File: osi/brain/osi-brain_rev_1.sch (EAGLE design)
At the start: 8 parts, among them IC1 TINY24/44/84-PU

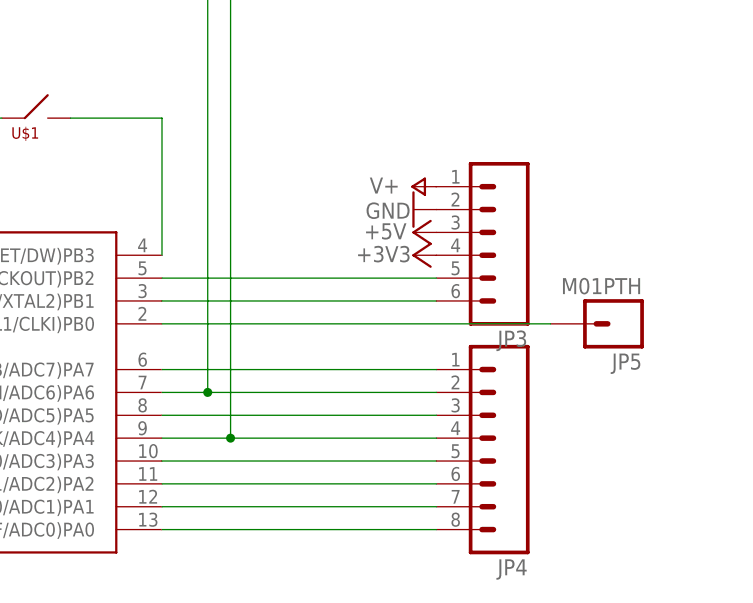
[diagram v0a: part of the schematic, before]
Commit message: power-ac
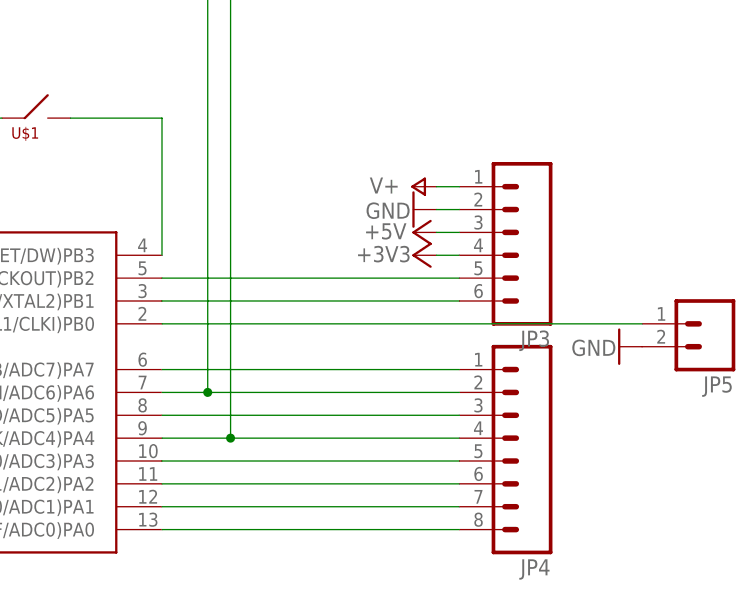
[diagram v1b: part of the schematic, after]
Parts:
- JP3: device SparkFun_mod:M06SIP -> SparkFun:M06SIP
- JP4: device SparkFun_mod:M081X08 -> SparkFun:M081X08
- JP5: value M01PTH -> (none); device SparkFun_mod:M01PTH -> SparkFun_mod:M021X02_NO_SILK
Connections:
- net GND: now also JP5.2
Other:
- moved on the sheet: JP3, JP4
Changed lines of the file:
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@@
 <part name="GND2" library="SparkFun" deviceset="GND" device=""/>
 <part name="GND5" library="SparkFun" deviceset="GND" device=""/>
-<part name="JP3" library="SparkFun_mod" deviceset="M06" device="SIP"/>
-<part name="JP4" library="SparkFun_mod" deviceset="M08" device="1X08"/>
 <part name="GND4" library="SparkFun" deviceset="GND" device=""/>
 <part name="P+2" library="supply1" deviceset="V+" device=""/>
@@
 <part name="JP2" library="SparkFun_mod" deviceset="M05" device="PTH"/>
 <part name="P+4" library="supply1" deviceset="+5V" device=""/>
-<part name="JP5" library="SparkFun_mod" deviceset="M01" device="PTH"/>
 <part name="+3V2" library="supply1" deviceset="+3V3" device=""/>
+<part name="JP3" library="SparkFun" deviceset="M06" device="SIP"/>
+<part name="JP4" library="SparkFun" deviceset="M08" device="1X08"/>
+<part name="GND3" library="SparkFun" deviceset="GND" device=""/>
+<part name="JP5" library="SparkFun_mod" deviceset="M02" device="1X02_NO_SILK"/>
 </parts>
 <sheets>
@@
 <attribute name="VALUE" x="111.506" y="67.564" size="1.778" layer="96"/>
 </instance>
-<instance part="JP3" gate="G$1" x="124.46" y="66.04" rot="R180"/>
-<instance part="JP4" gate="G$1" x="124.46" y="43.18" rot="R180"/>
 <instance part="GND4" gate="1" x="93.98" y="121.92" rot="R180"/>
 <instance part="P+2" gate="1" x="116.84" y="71.12" smashed="yes" rot="R90">
@@
 <attribute name="VALUE" x="105.156" y="122.682" size="1.778" layer="96" rot="R90"/>
 </instance>
-<instance part="JP5" gate="G$1" x="139.7" y="55.88" rot="R180"/>
 <instance part="+3V2" gate="G$1" x="22.86" y="45.72" smashed="yes" rot="R90">
 <attribute name="VALUE" x="22.606" y="46.736" size="1.778" layer="96" rot="R180"/>
 </instance>
+<instance part="JP3" gate="G$1" x="127" y="66.04" rot="R180"/>
+<instance part="JP4" gate="G$1" x="127" y="43.18" rot="R180"/>
+<instance part="GND3" gate="1" x="139.7" y="53.34" smashed="yes" rot="R270">
+<attribute name="VALUE" x="134.366" y="52.324" size="1.778" layer="96"/>
+</instance>
+<instance part="JP5" gate="G$1" x="149.86" y="55.88" rot="R180"/>
 </instances>
 <busses>
@@
 </segment>
 <segment>
+<pinref part="GND5" gate="1" pin="GND"/>
+<wire x1="121.92" y1="68.58" x2="119.38" y2="68.58" width="0.1524" layer="91"/>
 <pinref part="JP3" gate="G$1" pin="2"/>
-<pinref part="GND5" gate="1" pin="GND"/>
+</segment>
+<segment>
+<pinref part="GND3" gate="1" pin="GND"/>
+<pinref part="JP5" gate="G$1" pin="2"/>
 </segment>
 </net>
@@
 <segment>
 <pinref part="IC1" gate="1" pin="(PCINT3/T0/ADC3)PA3"/>
-<wire x1="119.38" y1="40.64" x2="88.9" y2="40.64" width="0.1524" layer="91"/>
+<wire x1="121.92" y1="40.64" x2="88.9" y2="40.64" width="0.1524" layer="91"/>
 <pinref part="JP4" gate="G$1" pin="5"/>
 </segment>
@@
 <segment>
 <pinref part="IC1" gate="1" pin="(PCINT2/AIN1/ADC2)PA2"/>
-<wire x1="119.38" y1="38.1" x2="88.9" y2="38.1" width="0.1524" layer="91"/>
+<wire x1="121.92" y1="38.1" x2="88.9" y2="38.1" width="0.1524" layer="91"/>
 <pinref part="JP4" gate="G$1" pin="6"/>
 </segment>
@@
 <segment>
 <pinref part="IC1" gate="1" pin="(PCINT1/AIN0/ADC1)PA1"/>
-<wire x1="119.38" y1="35.56" x2="88.9" y2="35.56" width="0.1524" layer="91"/>
+<wire x1="121.92" y1="35.56" x2="88.9" y2="35.56" width="0.1524" layer="91"/>
 <pinref part="JP4" gate="G$1" pin="7"/>
 </segment>
@@
 <segment>
 <pinref part="IC1" gate="1" pin="(PCINT0/AREF/ADC0)PA0"/>
-<wire x1="119.38" y1="33.02" x2="88.9" y2="33.02" width="0.1524" layer="91"/>
+<wire x1="121.92" y1="33.02" x2="88.9" y2="33.02" width="0.1524" layer="91"/>
 <pinref part="JP4" gate="G$1" pin="8"/>
 </segment>
@@
 <segment>
 <wire x1="114.3" y1="109.22" x2="93.98" y2="109.22" width="0.1524" layer="91"/>
-<pinref part="JP4" gate="G$1" pin="2"/>
-<wire x1="93.98" y1="48.26" x2="119.38" y2="48.26" width="0.1524" layer="91"/>
+<wire x1="93.98" y1="48.26" x2="121.92" y2="48.26" width="0.1524" layer="91"/>
 <wire x1="93.98" y1="109.22" x2="93.98" y2="48.26" width="0.1524" layer="91"/>
 <junction x="93.98" y="48.26"/>
@@
 <pinref part="IC1" gate="1" pin="(PCINT6/OC1A/SDA/MOSI/ADC6)PA6"/>
 <wire x1="88.9" y1="48.26" x2="93.98" y2="48.26" width="0.1524" layer="91"/>
+<pinref part="JP4" gate="G$1" pin="2"/>
 </segment>
 </net>
 <net name="V+" class="0">
 <segment>
+<pinref part="P+2" gate="1" pin="V+"/>
+<wire x1="121.92" y1="71.12" x2="119.38" y2="71.12" width="0.1524" layer="91"/>
 <pinref part="JP3" gate="G$1" pin="1"/>
-<pinref part="P+2" gate="1" pin="V+"/>
 </segment>
 </net>
@@
 <segment>
 <pinref part="IC1" gate="1" pin="(PCINT5/OC1B/MISO/DO/ADC5)PA5"/>
+<wire x1="88.9" y1="45.72" x2="121.92" y2="45.72" width="0.1524" layer="91"/>
 <pinref part="JP4" gate="G$1" pin="3"/>
-<wire x1="88.9" y1="45.72" x2="119.38" y2="45.72" width="0.1524" layer="91"/>
 </segment>
 </net>
@@
 <segment>
 <wire x1="114.3" y1="106.68" x2="96.52" y2="106.68" width="0.1524" layer="91"/>
-<pinref part="JP4" gate="G$1" pin="4"/>
-<wire x1="96.52" y1="43.18" x2="119.38" y2="43.18" width="0.1524" layer="91"/>
+<wire x1="96.52" y1="43.18" x2="121.92" y2="43.18" width="0.1524" layer="91"/>
 <wire x1="96.52" y1="106.68" x2="96.52" y2="43.18" width="0.1524" layer="91"/>
 <wire x1="76.2" y1="106.68" x2="96.52" y2="106.68" width="0.1524" layer="91"/>
@@
 <wire x1="88.9" y1="43.18" x2="96.52" y2="43.18" width="0.1524" layer="91"/>
 <junction x="96.52" y="43.18"/>
+<pinref part="JP4" gate="G$1" pin="4"/>
 </segment>
 </net>
@@
 <segment>
 <pinref part="IC1" gate="1" pin="(PCINT10/INT0/OC0A/CKOUT)PB2"/>
-<wire x1="88.9" y1="60.96" x2="119.38" y2="60.96" width="0.1524" layer="91"/>
+<wire x1="88.9" y1="60.96" x2="121.92" y2="60.96" width="0.1524" layer="91"/>
 <pinref part="JP3" gate="G$1" pin="5"/>
 </segment>
@@
 <segment>
 <pinref part="IC1" gate="1" pin="(PCINT9/XTAL2)PB1"/>
-<wire x1="88.9" y1="58.42" x2="119.38" y2="58.42" width="0.1524" layer="91"/>
+<wire x1="88.9" y1="58.42" x2="121.92" y2="58.42" width="0.1524" layer="91"/>
 <pinref part="JP3" gate="G$1" pin="6"/>
 </segment>
@@
 <segment>
 <pinref part="IC1" gate="1" pin="(PCINT8/XTAL1/CLKI)PB0"/>
-<wire x1="88.9" y1="55.88" x2="132.08" y2="55.88" width="0.1524" layer="91"/>
+<wire x1="88.9" y1="55.88" x2="142.24" y2="55.88" width="0.1524" layer="91"/>
 <pinref part="JP5" gate="G$1" pin="1"/>
 </segment>
@@
 <segment>
 <pinref part="IC1" gate="1" pin="(PCINT7/ICP/OC0B/ADC7)PA7"/>
+<wire x1="88.9" y1="50.8" x2="121.92" y2="50.8" width="0.1524" layer="91"/>
 <pinref part="JP4" gate="G$1" pin="1"/>
-<wire x1="88.9" y1="50.8" x2="119.38" y2="50.8" width="0.1524" layer="91"/>
 </segment>
 </net>
@@
 </segment>
 <segment>
+<pinref part="+3V4" gate="G$1" pin="+3V3"/>
+<wire x1="121.92" y1="63.5" x2="119.38" y2="63.5" width="0.1524" layer="91"/>
 <pinref part="JP3" gate="G$1" pin="4"/>
-<pinref part="+3V4" gate="G$1" pin="+3V3"/>
 </segment>
 <segment>
@@
 <net name="+5V" class="0">
 <segment>
+<pinref part="P+3" gate="1" pin="+5V"/>
+<wire x1="121.92" y1="66.04" x2="119.38" y2="66.04" width="0.1524" layer="91"/>
 <pinref part="JP3" gate="G$1" pin="3"/>
-<pinref part="P+3" gate="1" pin="+5V"/>
-</segment>
-<segment>
+</segment>
+<segment>
